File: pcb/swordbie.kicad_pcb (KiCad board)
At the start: 2 copper layers, 60.5 x 60 mm, 14 parts, among them J1 Conn_01x08_Pin, J2 Conn_01x04_Pin, SW1 SW_Push, SW2 SW_Push, U1 XIAO-ESP32-C3-SMD, U2 DHT11

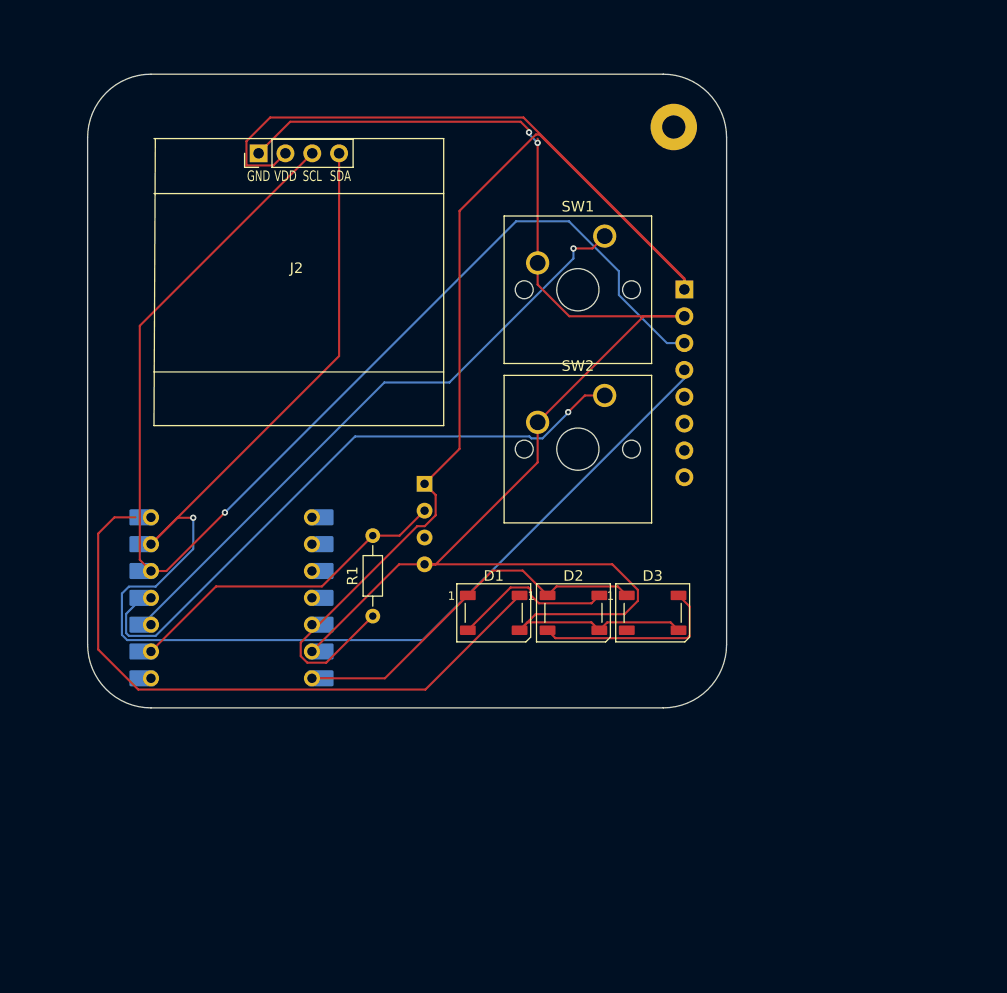
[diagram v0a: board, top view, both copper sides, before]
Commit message: new pcb files updated design
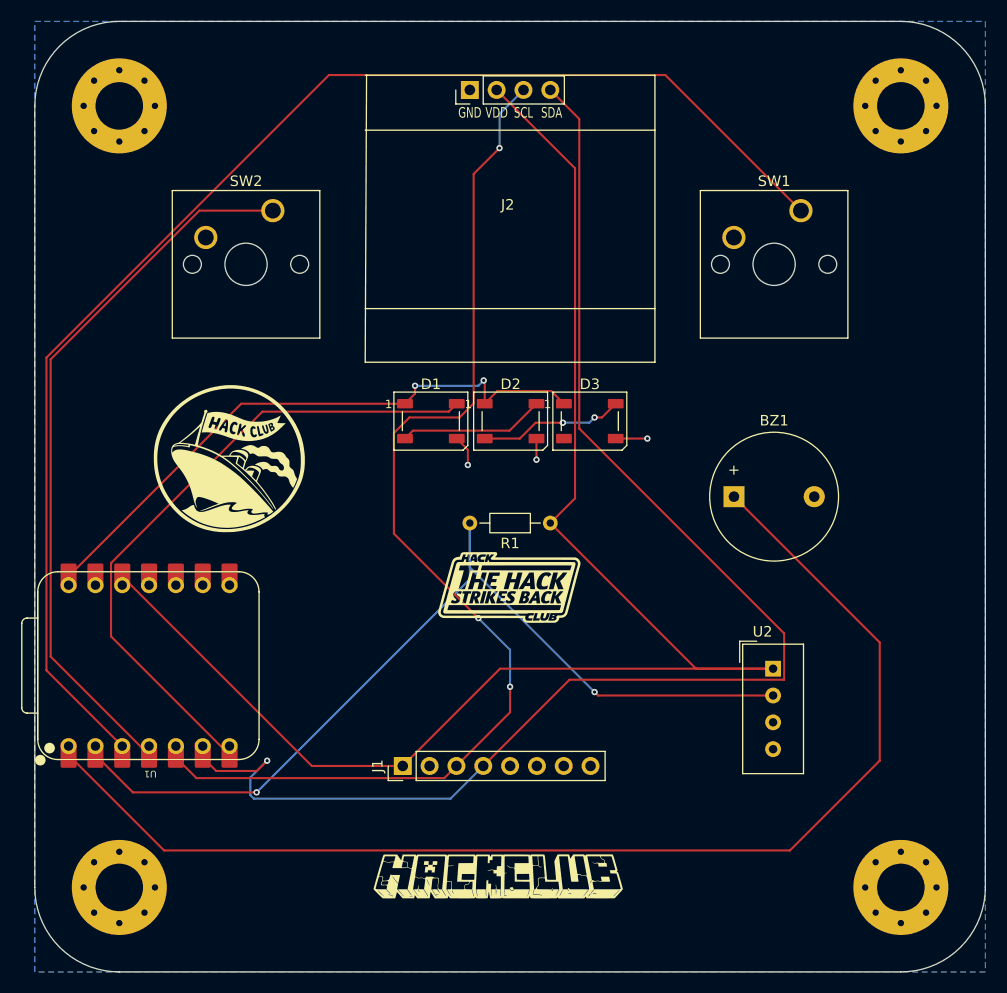
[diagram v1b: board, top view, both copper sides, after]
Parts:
- removed the REF** at (80.5, 30.0)
- added BZ1: Buzzer, Buzzer_Beeper:Buzzer_12x9.5RM7.6, F.Cu at (86.2, 65.0)
- added G***: LOGO, LOGO, F.Cu at (65.0, 73.5)
- added G***: LOGO, LOGO, F.Cu at (38.5, 61.5)
- added G***: LOGO, LOGO, F.Cu at (64.0, 101.0)
- added G***: LOGO, LOGO, B.Cu at (62.5, 91.5)
- added G***: LOGO, LOGO, B.Cu at (46.5, 64.5)
- added REF**: MountingHole_4.5mm_Pad_Via, MountingHole:MountingHole_4.5mm_Pad_Via, F.Cu at (28.0, 28.0)
- added REF**: MountingHole_4.5mm_Pad_Via, MountingHole:MountingHole_4.5mm_Pad_Via, F.Cu at (28.0, 102.0)
- added REF**: MountingHole_4.5mm_Pad_Via, MountingHole:MountingHole_4.5mm_Pad_Via, F.Cu at (102.0, 102.0)
- added REF**: MountingHole_4.5mm_Pad_Via, MountingHole:MountingHole_4.5mm_Pad_Via, F.Cu at (102.0, 28.0)
- J1, U1, U2: moved to F.Cu
- moved G*** 64.1 mm to (98.5, 49.5), turned to 180 degrees
- moved J1 52.4 mm to (54.8, 90.5), turned to 90 degrees
- moved U2 37.4 mm to (89.9, 81.3), turned to 0 degrees
- moved SW2 36.0 mm to (42.5, 37.9)
- moved J2 20.9 mm to (65.0, 26.5)
- moved G*** 20.2 mm to (91.0, 65.5), turned to 180 degrees
- moved D1 19.1 mm to (57.5, 57.9)
- moved D2 19.1 mm to (65.0, 57.9)
- moved D3 19.1 mm to (72.5, 57.9)
- moved R1 19.0 mm to (68.8, 67.5), turned to 180 degrees
- moved SW1 18.7 mm to (92.5, 37.9)
- moved G*** 11.7 mm to (66.0, 37.5), turned to 180 degrees
- moved U1 10.1 mm to (30.8, 81.0), turned to 180 degrees
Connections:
- U1 pad 1: unconnected-(U1-D0-Pad1) -> /GPI00
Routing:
- net GND: track 159.2 -> 7.93 mm, vias 2 -> 3
- net /GPI00: track 0.00 -> 114.8 mm
- net /GPI02: track 59.6 -> 127.6 mm, vias 1 -> 0
- net /DHT11 DATA: track 31.4 -> 88.5 mm, vias 0 -> 2
- net /5V: track 35.7 -> 58.2 mm, vias 0 -> 2
- net /SCL: track 117.1 -> 107.5 mm, vias 1 -> 3
- net /GPI03: track 59.0 -> 68.2 mm, vias 1 -> 0
- net Net-(D2-DOUT): track 18.1 -> 13.8 mm, vias 0 -> 2
- net /SDA: track 129.3 -> 132.4 mm
- net Net-(D1-DOUT): track 15.4 -> 13.8 mm
- net /DIN: track 60.3 -> 61.8 mm
- net +3.3V: track 145.7 -> 144.7 mm
- added copper zone on B.Cu, net GND
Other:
- board size 60.5 x 60 mm -> 90 x 90 mm
